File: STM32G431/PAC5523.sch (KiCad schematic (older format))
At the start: 90 parts, among them J1 W, J2 U, J3 V, U1 STM32G431CBUx, U10 MIC4605, U12 AMS1117-3.3, U4 XL7015, U6 MIC4605, U7 MIC4605, Y1 8Mhz

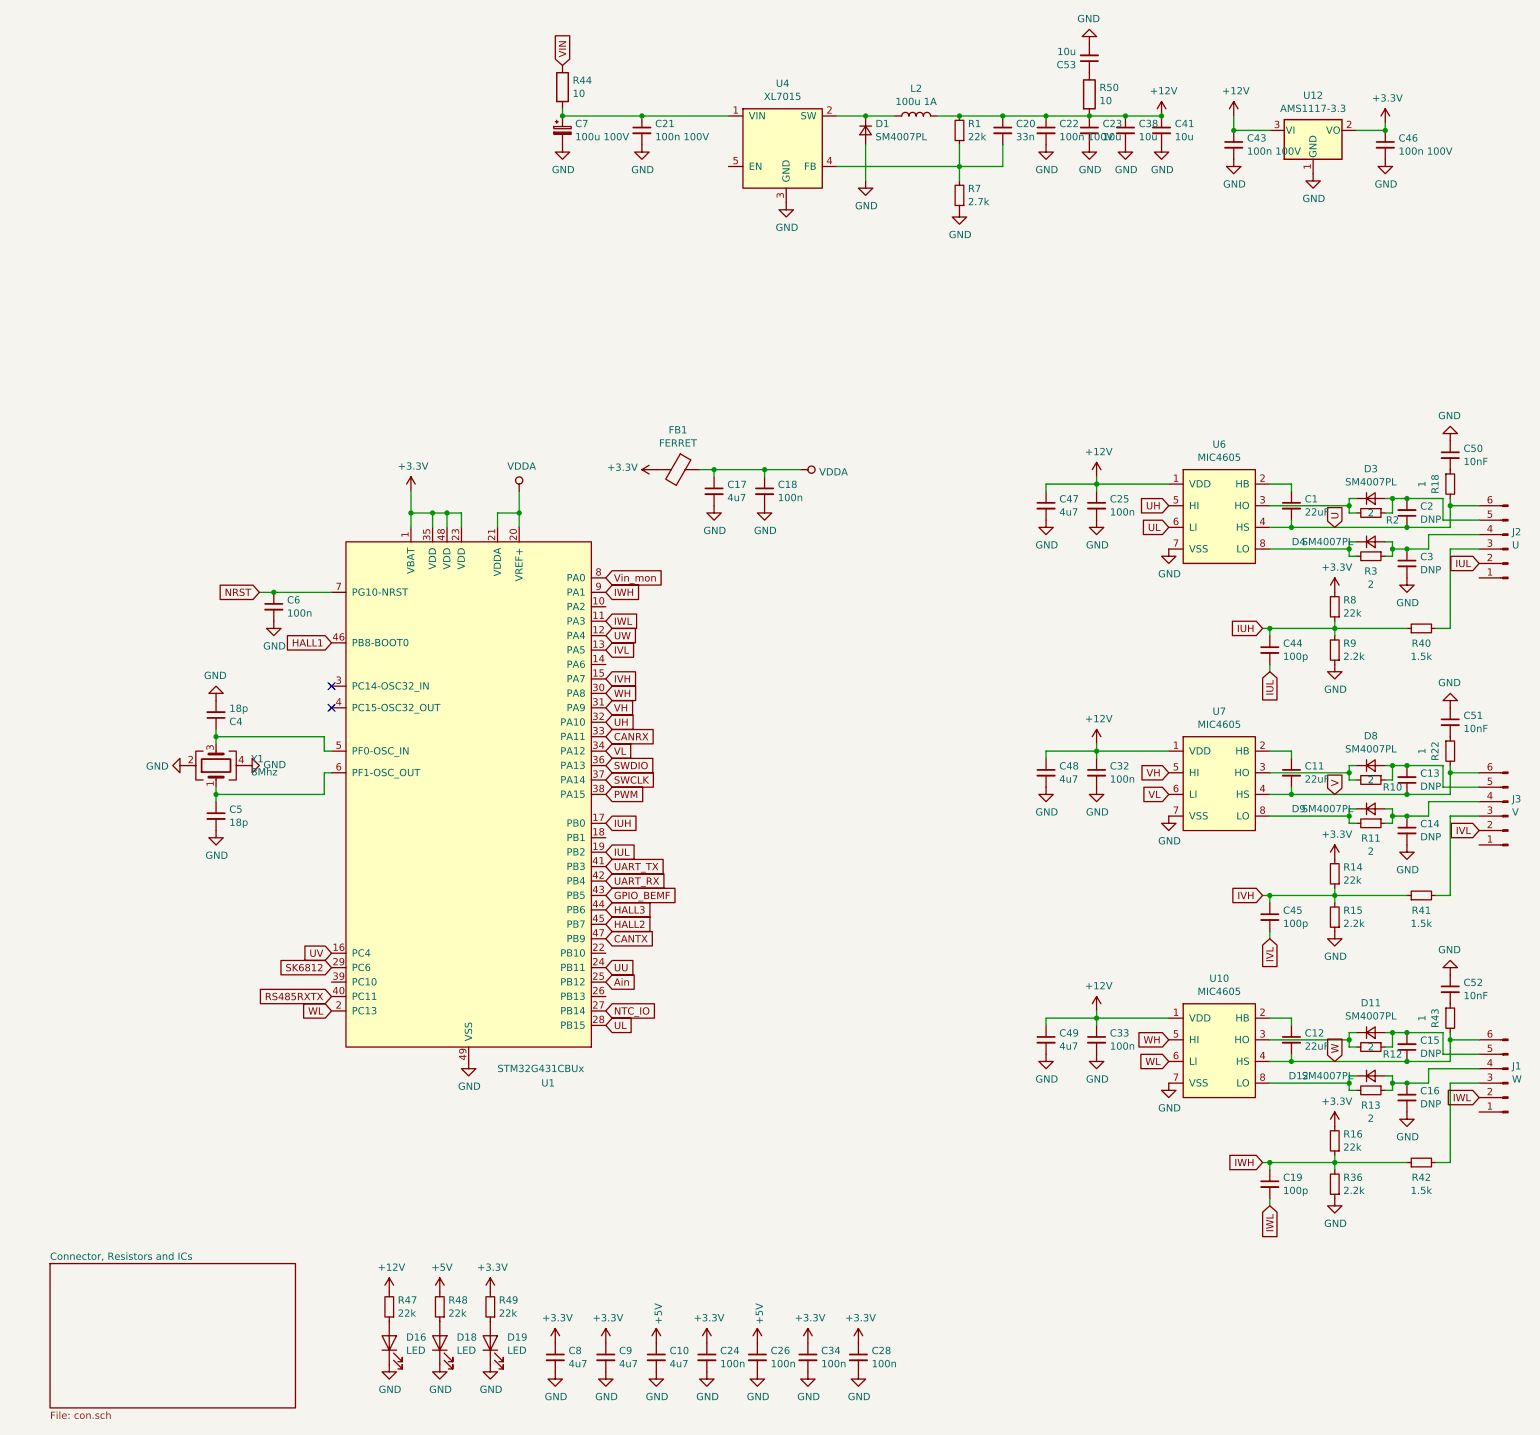
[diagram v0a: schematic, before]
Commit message: updated pcb
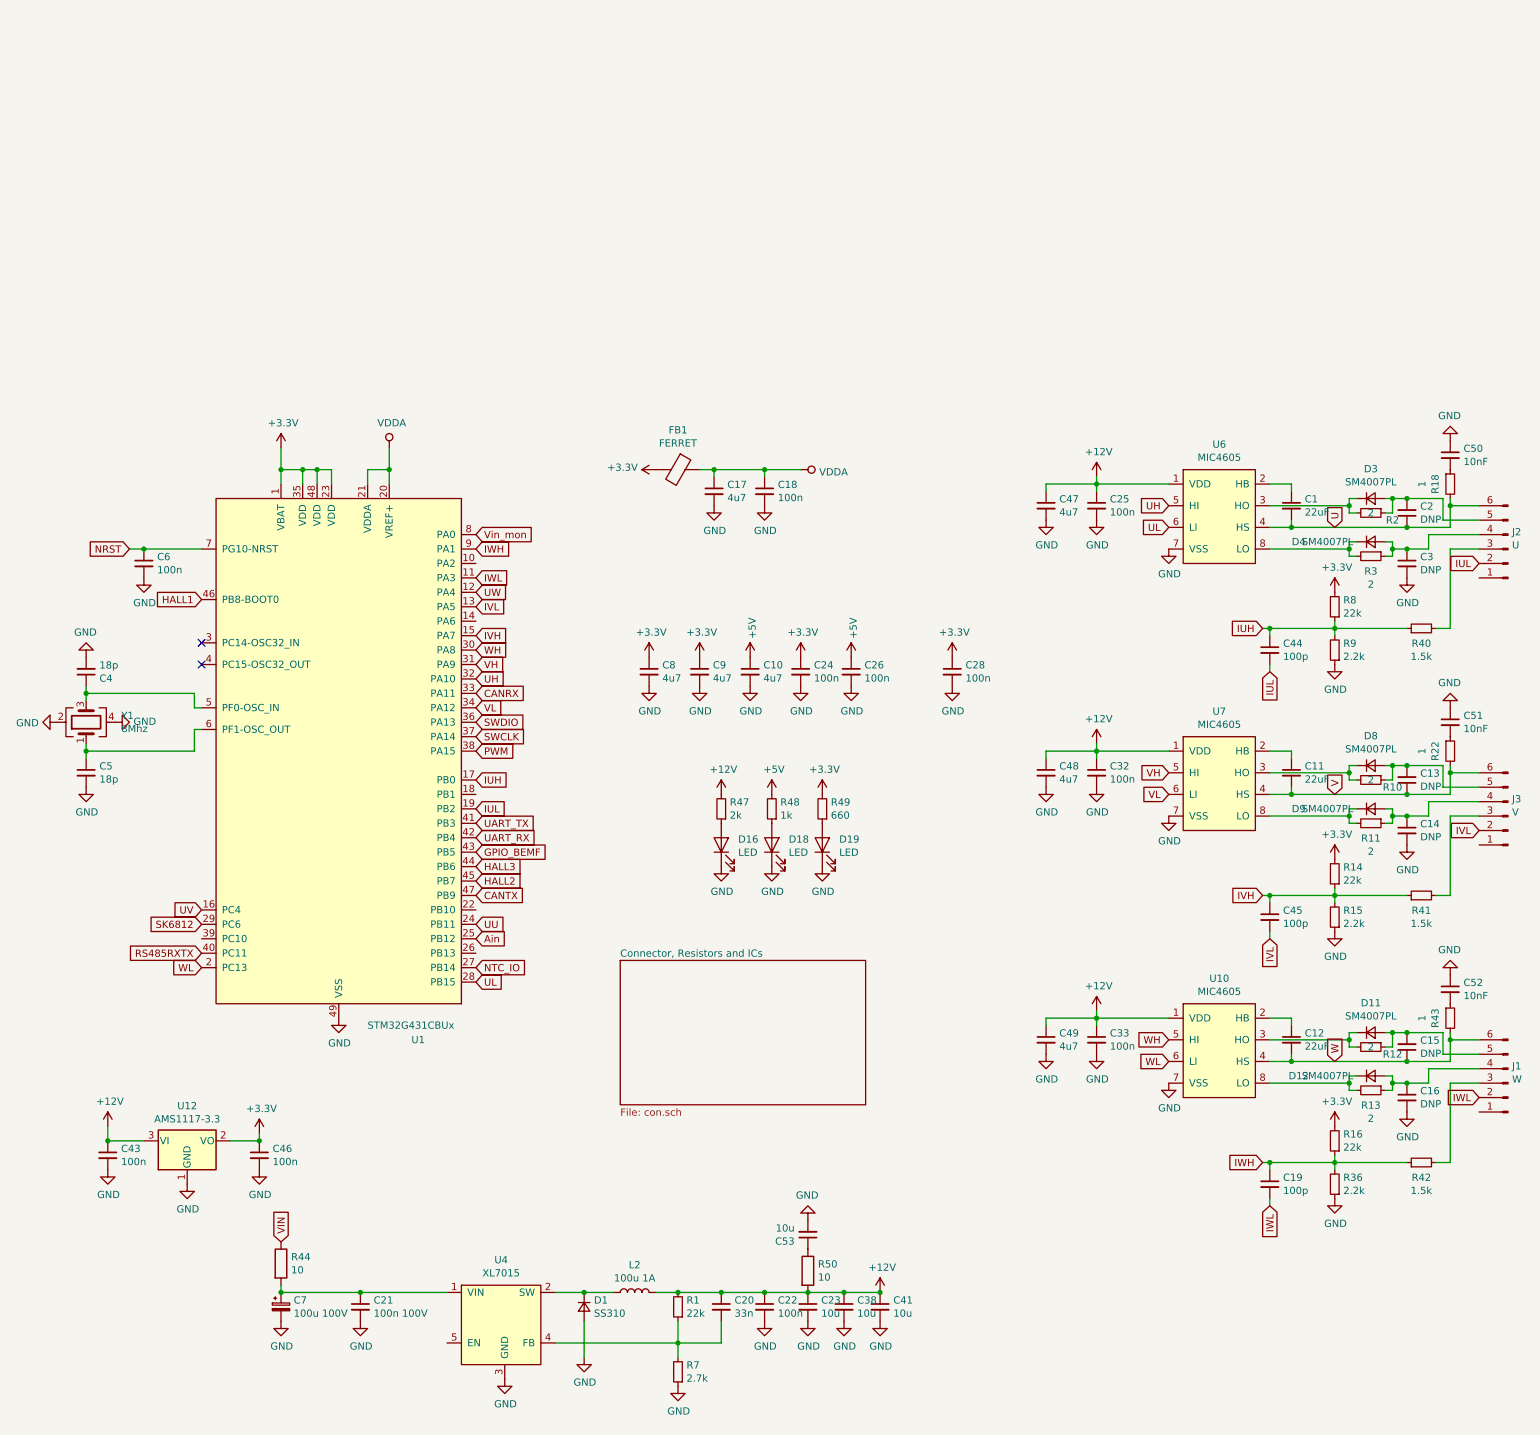
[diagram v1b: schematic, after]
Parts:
- removed C34: 100n, Capacitor_SMD:C_0603_1608Metric, symbol Device:C_Small
- C22, C43, C46: value 100n 100V -> 100n
- D1: value SM4007PL -> SS310; footprint Diode_SMD:D_SOD-123F -> Diode_SMD:D_SMA; LCSC (none) -> C14996
- R47: value 22k -> 2k
- R48: value 22k -> 1k
- R49: value 22k -> 660
- U1: footprint Package_DFN_QFN:QFN-48-1EP_6x6mm_P0.4mm_EP4.2x4.2mm -> Package_DFN_QFN:QFN-48-1EP_7x7mm_P0.5mm_EP5.3x5.3mm
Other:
- moved on the sheet: C10, C20, C21, C22, C23, C24, C26, C28, C38, C4, C41, C43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
